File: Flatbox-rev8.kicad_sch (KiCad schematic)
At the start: 72 parts, among them SW1 SW_Push, SW10 GPIO18, SW11 GPIO25, SW12 GPIO27, SW13 GPIO29, SW14 GPIO19, SW15 GPIO24, SW16 GPIO26, SW17 GPIO28, SW18 GPIO16, SW19 SW_Push, SW2 SW_Push, SW20 SW_Push, SW21 GPIO16, SW3 SW_Push, SW4 SW_Push, SW5 SW_Push, SW6 SW_Push, SW7 GPIO9, SW8 GPIO10, SW9 GPIO11, U1 RP2350_60QFN, U2 TLV73333PDBV, U3 W25Q128JVS, Y1 ABM8-272-T3

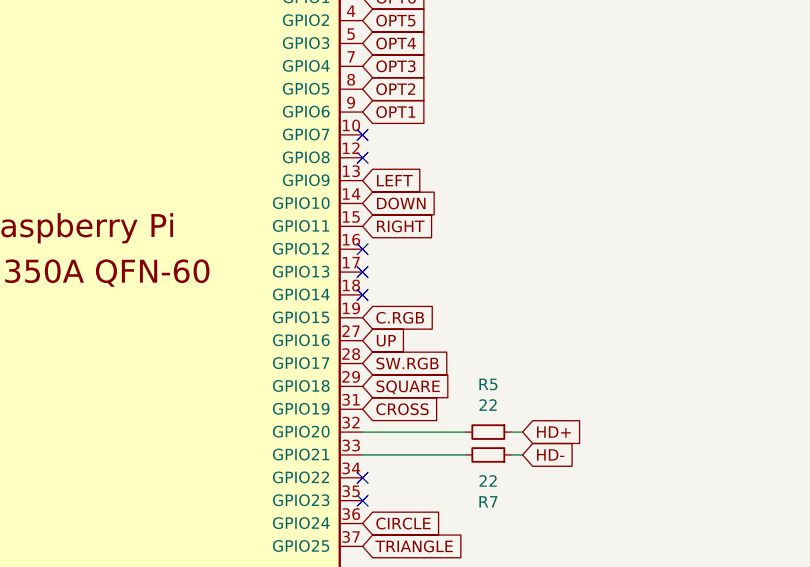
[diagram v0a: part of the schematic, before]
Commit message: final design inshallah
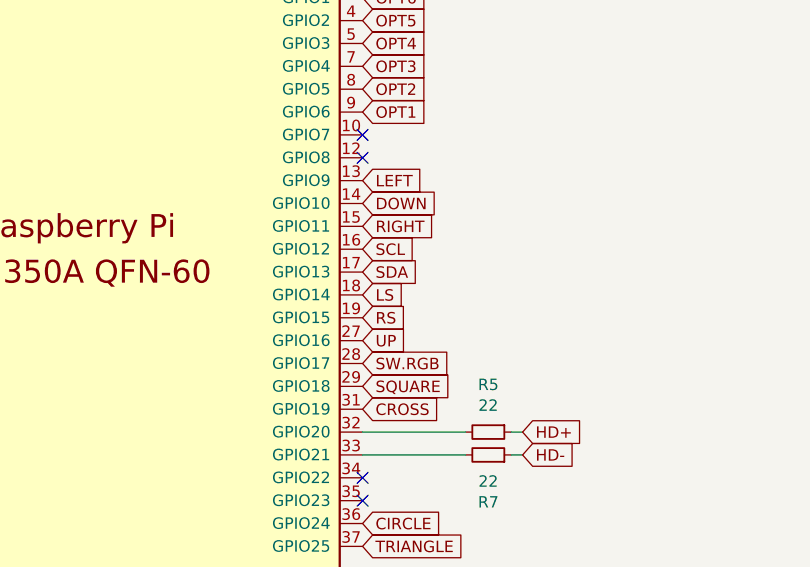
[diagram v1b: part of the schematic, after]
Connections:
- net SCL: now reaches U1.16 (GPIO12)
- net SDA: now reaches U1.17 (GPIO13)
- net LS: now reaches U1.18 (GPIO14)
- net C.RGB renamed RS
- no-connect marks 11 -> 8
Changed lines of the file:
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@@
-	)
-	(no_connect
-		(at 269.24 123.19)
 	)
 	(no_connect
@@
 	)
 	(no_connect
-		(at 269.24 125.73)
-	)
-	(no_connect
 		(at 269.24 110.49)
 	)
@@
 	)
 	(no_connect
-		(at 269.24 120.65)
-	)
-	(no_connect
 		(at 110.49 231.14)
 	)
@@
 		)
 	)
-	(global_label "C.RGB"
+	(global_label "RS"
 		(shape input)
 		(at 269.24 128.27 0)
@@
 		)
 		(property "Intersheetrefs" "${INTERSHEET_REFS}"
-			(at 277.2558 128.27 0)
+			(at 274.0505 128.27 0)
 			(effects
 				(font
@@
 		)
 	)
+	(global_label "SDA"
+		(shape input)
+		(at 269.24 123.19 0)
+		(fields_autoplaced yes)
+		(effects
+			(font
+				(size 1.27 1.27)
+			)
+			(justify left)
+		)
+		(property "Intersheetrefs" "${INTERSHEET_REFS}"
+			(at 275.1391 123.19 0)
+			(effects
+				(font
+					(size 1.27 1.27)
+				)
+				(justify left)
+				(hide yes)
+			)
+		)
+	)
 	(global_label "CROSS"
 		(shape input)
@@
 		)
 	)
+	(global_label "LS"
+		(shape input)
+		(at 269.24 125.73 0)
+		(fields_autoplaced yes)
+		(effects
+			(font
+				(size 1.27 1.27)
+			)
+			(justify left)
+		)
+		(property "Intersheetrefs" "${INTERSHEET_REFS}"
+			(at 273.8086 125.73 0)
+			(effects
+				(font
+					(size 1.27 1.27)
+				)
+				(justify left)
+				(hide yes)
+			)
+		)
+	)
 	(global_label "UP"
 		(shape input)
@@
 			(effects
 				(font
+					(size 1.27 1.27)
+				)
+				(justify left)
+				(hide yes)
+			)
+		)
+	)
+	(global_label "SCL"
+		(shape input)
+		(at 269.24 120.65 0)
+		(fields_autoplaced yes)
+		(effects
+			(font
+				(size 1.27 1.27)
+			)
+			(justify left)
+		)
+		(property "Intersheetrefs" "${INTERSHEET_REFS}"
+			(at 275.0786 120.65 0)
+			(effects
+				(font
